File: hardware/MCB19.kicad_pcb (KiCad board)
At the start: 2 copper layers, 172.8 x 81.5 mm, 118 parts, among them J401 USART, J402 DISABLE, J601 RJ45, J602 RJ45, J611 +BAT_IN, J612 -BAT_IN, J613 +BAT_OUT, J614 -BAT_OUT, Q601 IRFP260N, Q602 IRFP260N, Q603 BC857, Q604 BC847, U201 MCP2551-I/SN, U202 MCP2515-xSO, U301 LM7805, U401 ATMEGA328P-PU, U501 LM7812, U601 LM5104MNOPB, U602 INA240A4D, U603 LM324, Y201 16MHz, Y401 16MHz

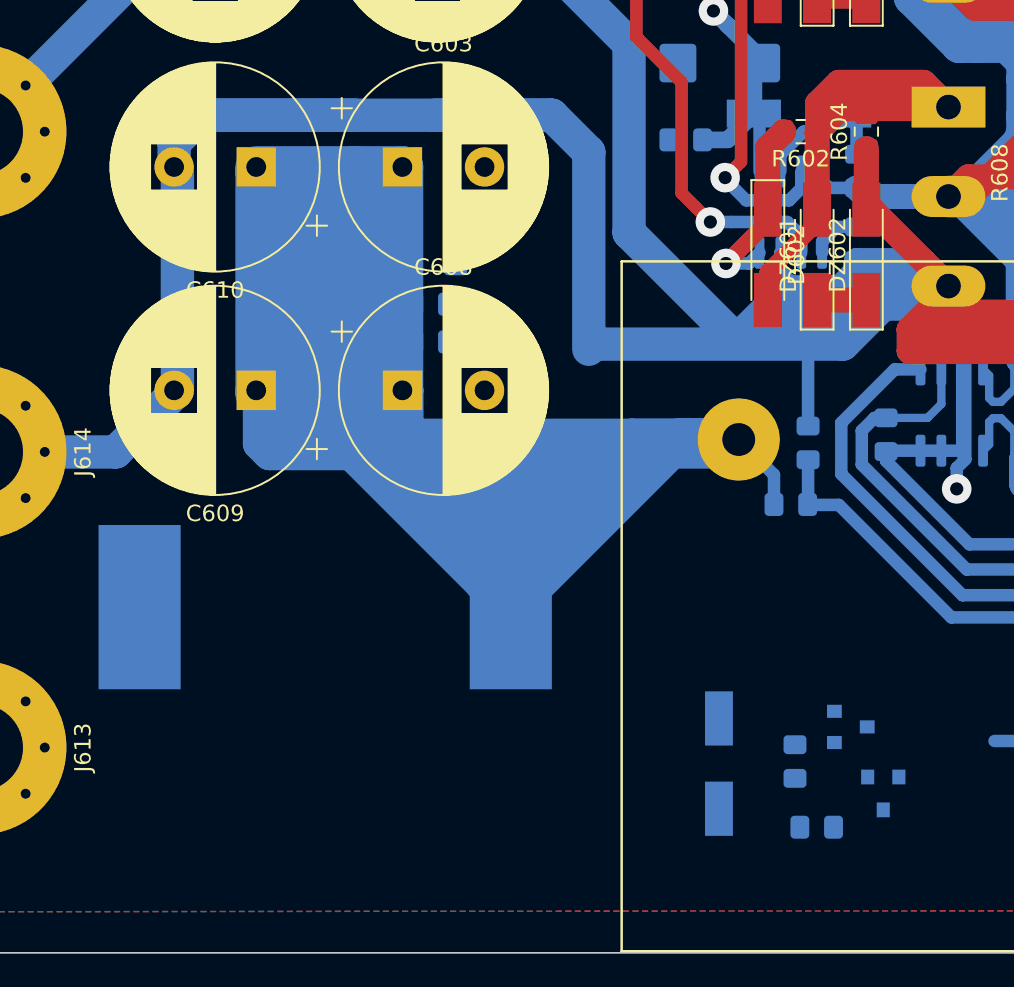
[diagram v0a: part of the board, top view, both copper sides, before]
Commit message: relay driver almost finished
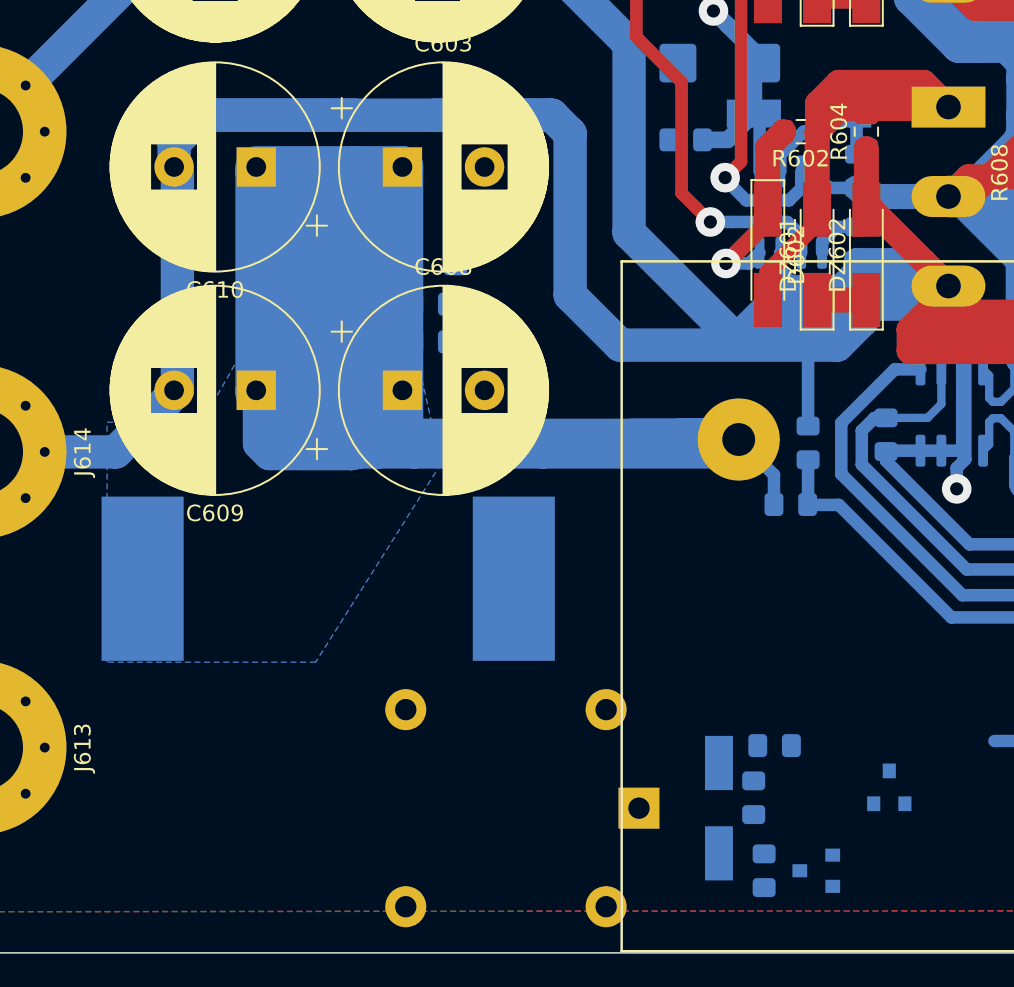
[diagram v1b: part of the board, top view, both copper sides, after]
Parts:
- added K601: G5LE-1, Relay_THT:Relay_SPDT_Omron-G5LE-1, B.Cu at (97.2, 123.2)
- added R1: 90R, Resistor_SMD:R_0805_2012Metric_Pad1.15x1.40mm_HandSolder, B.Cu at (104.8, 127.0)
- moved F602 22.9 mm to (89.5, 109.2), turned to 180 degrees
- moved Q603 6.23 mm to (108.0, 127.0), turned to 180 degrees
- moved Q604 4.36 mm to (112.4, 121.9), turned to 90 degrees
- moved R612 4.23 mm to (104.1, 122.6), turned to 270 degrees
- moved D606 2.72 mm to (102.0, 123.2)
- moved R611 1.58 mm to (105.4, 119.4), turned to 0 degrees
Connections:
- F501 pad 2: /CANBUS CONN/CAN_18V -> VCC
- F602 pad 1: (no net) -> Net-(F602-Pad1)
- J601 pad 4: /CANBUS CONN/CAN_18V -> VCC
- J601 pad 5: /CANBUS CONN/CAN_18V -> VCC
- J602 pad 4: /CANBUS CONN/CAN_18V -> VCC
- J602 pad 5: /CANBUS CONN/CAN_18V -> VCC
- Q603 pad 2: (no net) -> VCC
- Q603 pad 3: /driver/relay_coil -> Net-(Q603-Pad3)
- U201 pad 5: (no net) -> Net-(U201-Pad5)
- U202 pad 10: (no net) -> Net-(U202-Pad10)
- U202 pad 11: (no net) -> Net-(U202-Pad11)
- U202 pad 3: (no net) -> Net-(U202-Pad3)
- U202 pad 4: (no net) -> Net-(U202-Pad4)
- U202 pad 5: (no net) -> Net-(U202-Pad5)
- U202 pad 6: (no net) -> Net-(U202-Pad6)
- U401 pad 12: (no net) -> Net-(U401-Pad12)
- U401 pad 26: (no net) -> Net-(U401-Pad26)
- U401 pad 27: (no net) -> Net-(U401-Pad27)
- U401 pad 28: (no net) -> Net-(U401-Pad28)
- U401 pad 5: (no net) -> Net-(U401-Pad5)
- U401 pad 6: (no net) -> Net-(U401-Pad6)
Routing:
- net Net-(C603-Pad1): track 352.3 -> 249.2 mm
- net VCC: track 0.00 -> 70.6 mm
- net /CANBUS CONN/CAN_18V: track 70.6 -> 0.00 mm
- net GND: track 914.6 -> 926.0 mm
- added copper zone on B.Cu, net Net-(C603-Pad1)
